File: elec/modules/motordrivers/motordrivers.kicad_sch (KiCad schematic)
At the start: 17 parts, among them IC2 VNH5019ATR-E, J1 Conn_01x02, J10 Conn_01x05, J2 Conn_01x05, J3 Conn_01x05, J9 Conn_01x05, Q1 AON6354

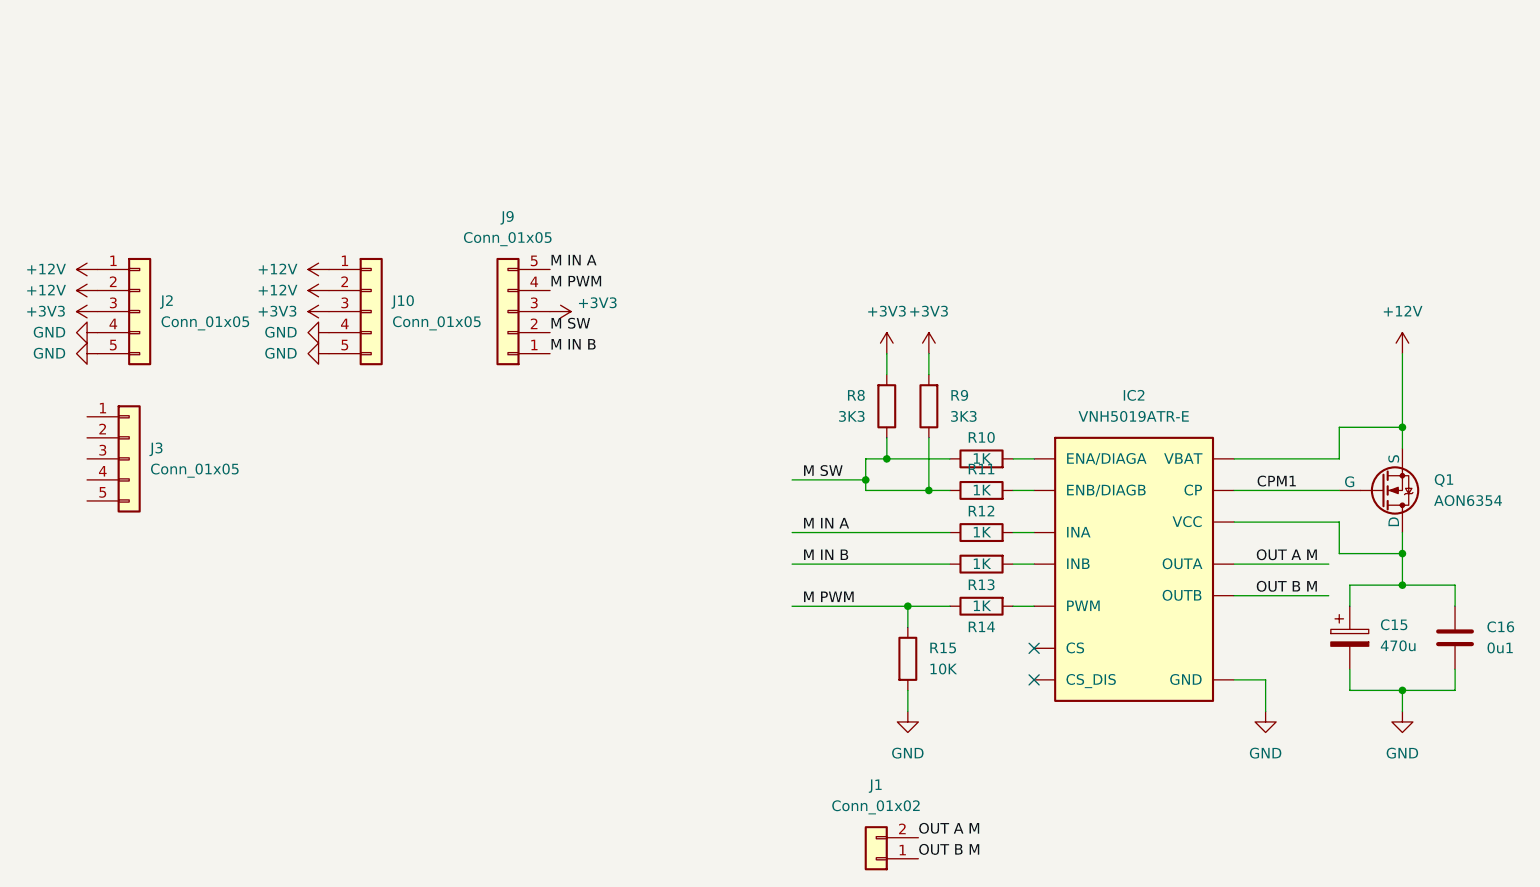
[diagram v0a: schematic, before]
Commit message: i think thats drivers done
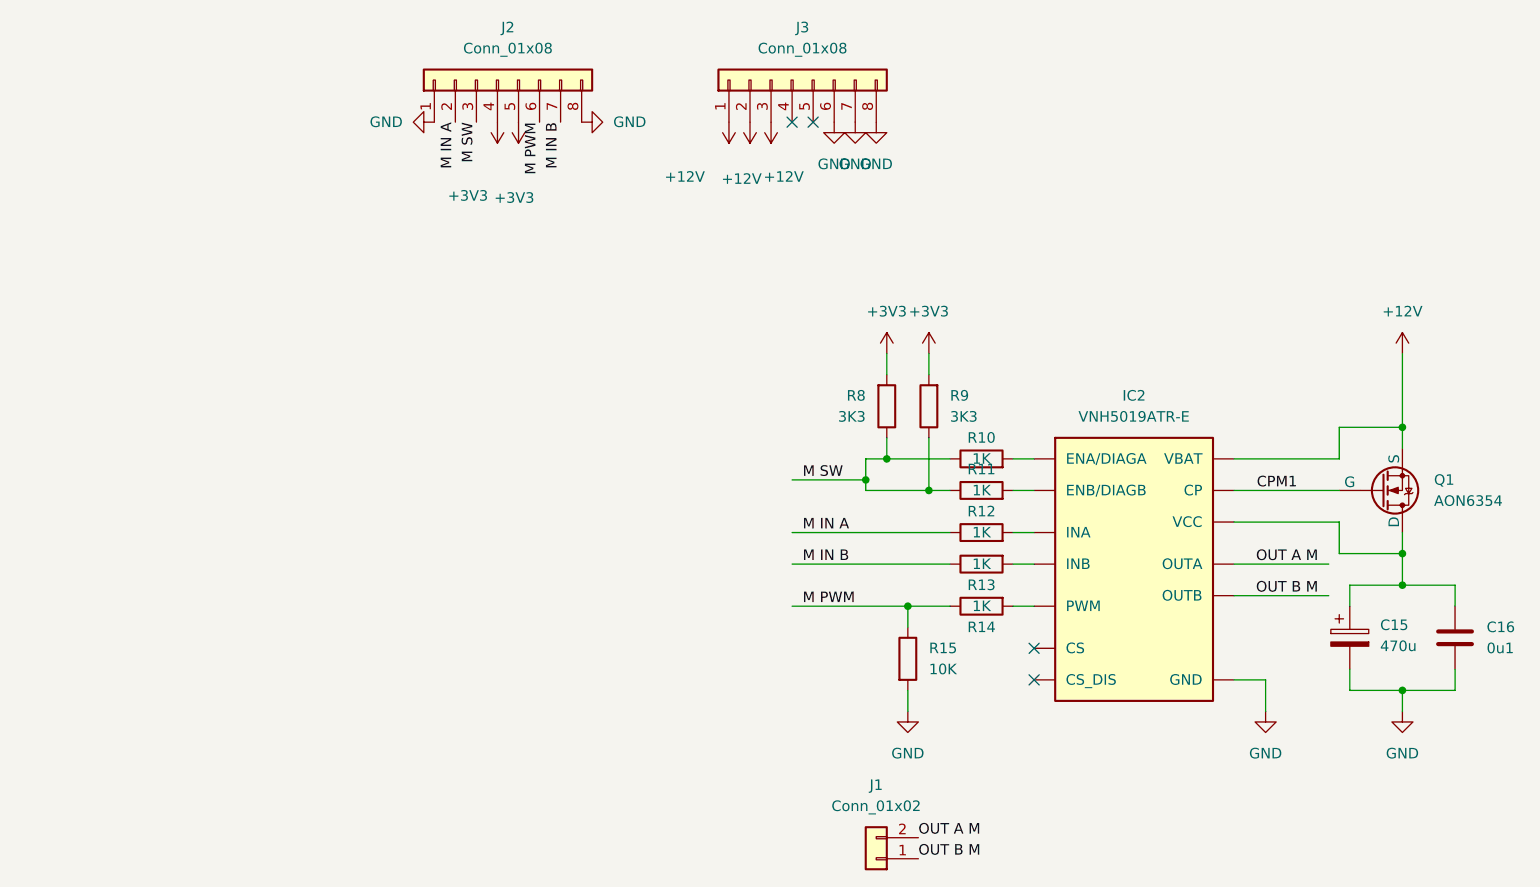
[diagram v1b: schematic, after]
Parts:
- removed J10, J2, J9: Conn_01x05, Pinheaders:PinHeader_1x05_P2.54mm_Vertical, symbol Connector_Generic:Conn_01x05
- removed J3: Conn_01x05, Connector_PinHeader_2.54mm:PinHeader_1x05_P2.54mm_Vertical, symbol Connector_Generic:Conn_01x05
- added J2, J3: Conn_01x08, Pinheaders:PinHeader_1x08_P2.54mm_Vertical, symbol Connector_Generic:Conn_01x08
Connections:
- net +12V: now also J3.1 (Pin_1), J3.2 (Pin_2), J3.3 (Pin_3)
- net +3V3: now also J2.4 (Pin_4), J2.5 (Pin_5)
- net GND: now also J2.1 (Pin_1), J2.8 (Pin_8), J3.6 (Pin_6), J3.7 (Pin_7), J3.8 (Pin_8)
- net M IN A: now also J2.2 (Pin_2)
- net M IN B: now also J2.7 (Pin_7)
- net M PWM: now also J2.6 (Pin_6)
- net M SW: now also J2.3 (Pin_3)
- no-connect marks 2 -> 4
